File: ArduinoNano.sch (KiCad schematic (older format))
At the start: 14 parts, among them IC601 ATMEGA328P-AU, IC602 FT232RL-TUBE, J601 M20-9980345, J602 USB_Connector, Y601 ECS-160-16-33B-CKM-TR

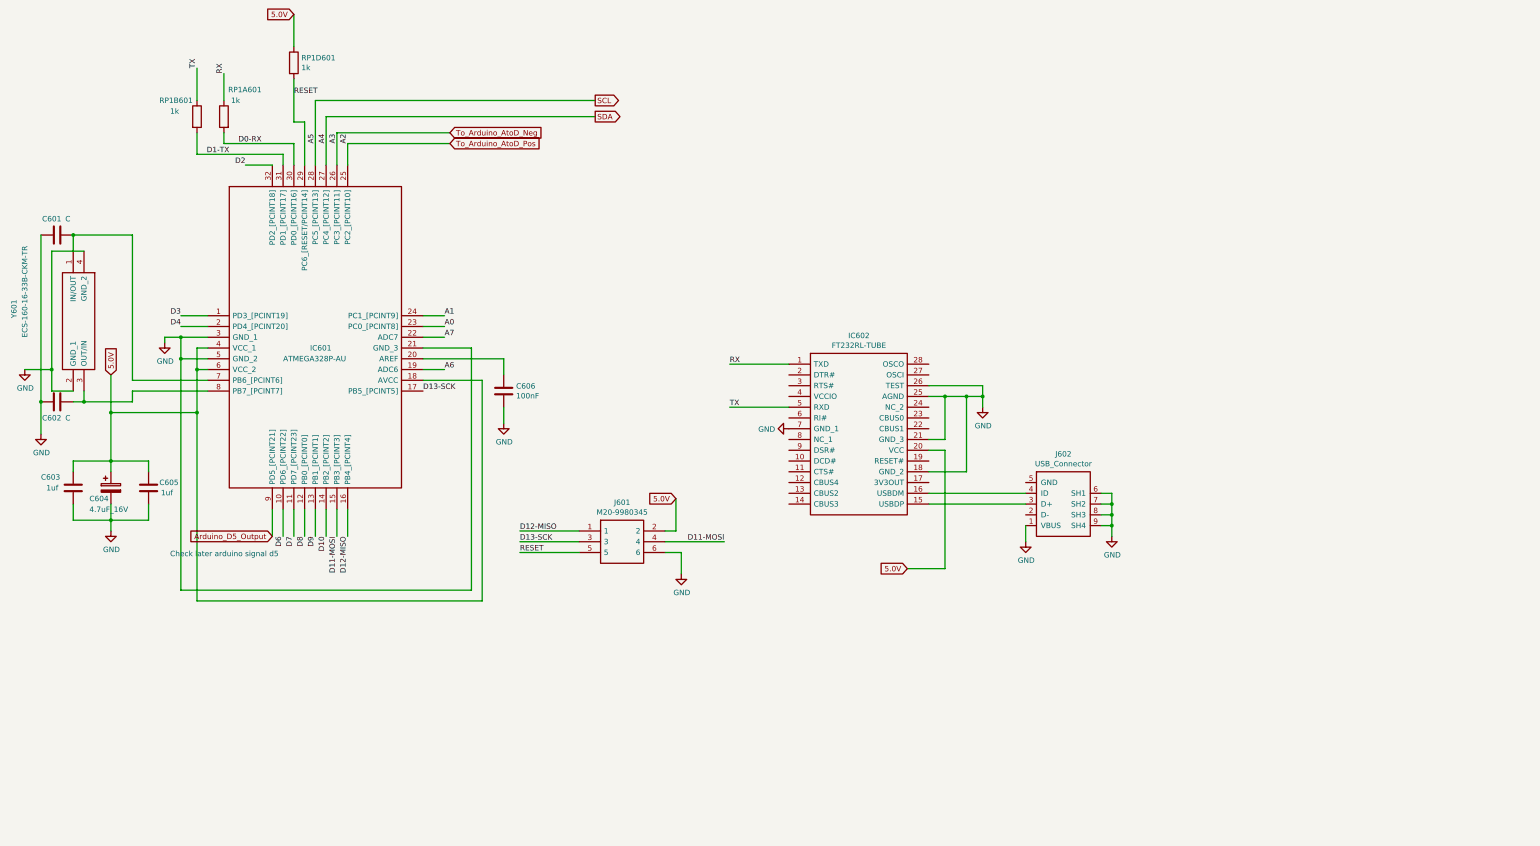
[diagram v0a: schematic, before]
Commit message: connect all grounds? maybe?
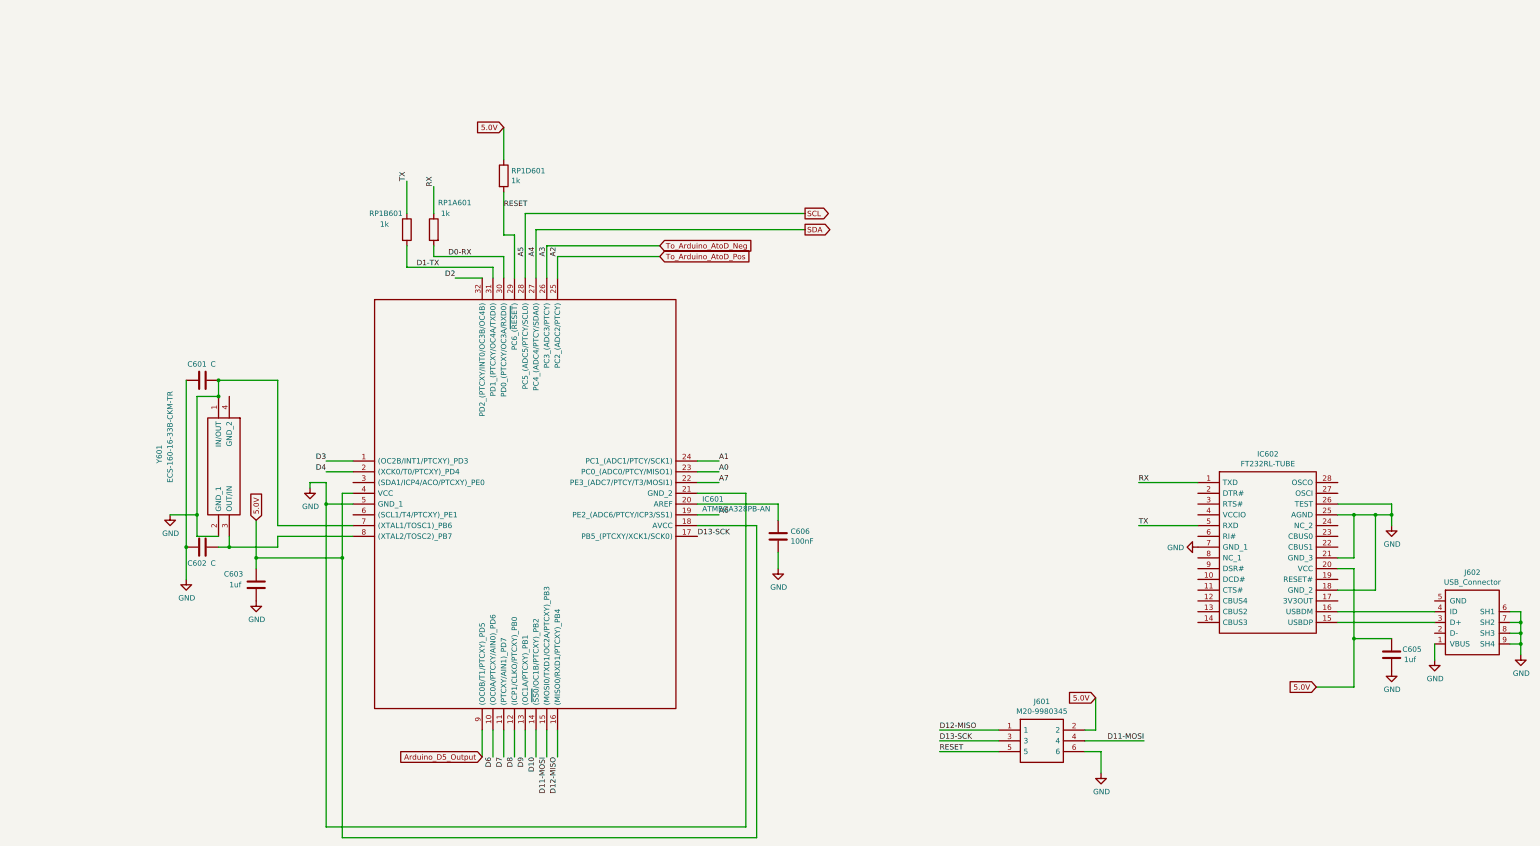
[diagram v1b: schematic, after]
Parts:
- removed C604: 4.7uF_16V, Capacitor_SMD:C_0402_1005Metric, symbol Device:CP
- removed IC601: ATMEGA328P-AU, footprint libraries:QFP80P900X900X120-32N, symbol ATMEGA328P-AU:ATMEGA328P-AU
- added IC601: ATMEGA328PB-AN, footprint libraries:QFP80P900X900X120-32N, symbol ATMEGA328PB-AN:ATMEGA328PB-AN
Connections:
- net 5.0V: now also IC601.18 (AVCC), IC601.4 (VCC)
- net A0: now also IC601.23 (PC0_(ADC0/PTCY/MISO1))
- net A1: now also IC601.24 (PC1_(ADC1/PTCY/SCK1))
- net A6: now also IC601.19 (PE2_(ADC6/PTCY/ICP3/SS1))
- net A7: now also IC601.22 (PE3_(ADC7/PTCY/T3/MOSI1))
- net Arduino_D5_Output: now also IC601.9 ((OC0B/T1/PTCXY)_PD5)
- net D0-RX: now also IC601.30 (PD0_(PTCXY/OC3A/RXD0))
- net D1-TX: now also IC601.31 (PD1_(PTCXY/OC4A/TXD0))
- net D10: now also IC601.14 ((~SS0~/OC1B/PTCXY)_PB2)
- net D11-MOSI: now also IC601.15 ((MOSI0/TXD1/OC2A/PTCXY)_PB3)
- net D12-MISO: now also IC601.16 ((MISO0/RXD1/PTCXY)_PB4)
- net D13-SCK: now also IC601.17 (PB5_(PTCXY/XCK1/SCK0))
- net D2: now also IC601.32 (PD2_(PTCXY/INT0/OC3B/OC4B))
- net D3: now also IC601.1 ((OC2B/INT1/PTCXY)_PD3)
- net D4: now also IC601.2 ((XCK0/T0/PTCXY)_PD4)
- net D6: now also IC601.10 ((OC0A/PTCXY/AIN0)_PD6)
- net D7: now also IC601.11 ((PTCXY/AIN1)_PD7)
- net D8: now also IC601.12 ((ICP1/CLKO/PTCXY)_PB0)
- net D9: now also IC601.13 ((OC1A/PTCXY)_PB1)
- net GND: now also C601.1, Y601.1 (IN/OUT), IC601.21 (GND_2), IC601.5 (GND_1), IC601.7 ((XTAL1/TOSC1)_PB6); no longer Y601.4 (GND_2)
- net RESET: now also IC601.29 (PC6_(~RESET))
- net SCL: now also IC601.28 (PC5_(ADC5/PTCY/SCL0))
- net SDA: now also IC601.27 (PC4_(ADC4/PTCY/SDA0))
- net To_Arduino_AtoD_Neg: now also IC601.26 (PC3_(ADC3/PTCY))
- net To_Arduino_AtoD_Pos: now also IC601.25 (PC2_(ADC2/PTCY))
- net at C602.1, Y601.3 (OUT/IN): now also IC601.8 ((XTAL2/TOSC2)_PB7)
- net at C606.1: now also IC601.20 (AREF)
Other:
- note removed: "Check later arduino signal d5"
- moved on the sheet: C601, C602, C603, C605, C606, IC602, J601, J602, RP1A601, RP1B601, RP1D601, Y601
